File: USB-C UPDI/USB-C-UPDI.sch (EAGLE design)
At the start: 9 parts, among them IC1 FT232RL, J2 61300511121

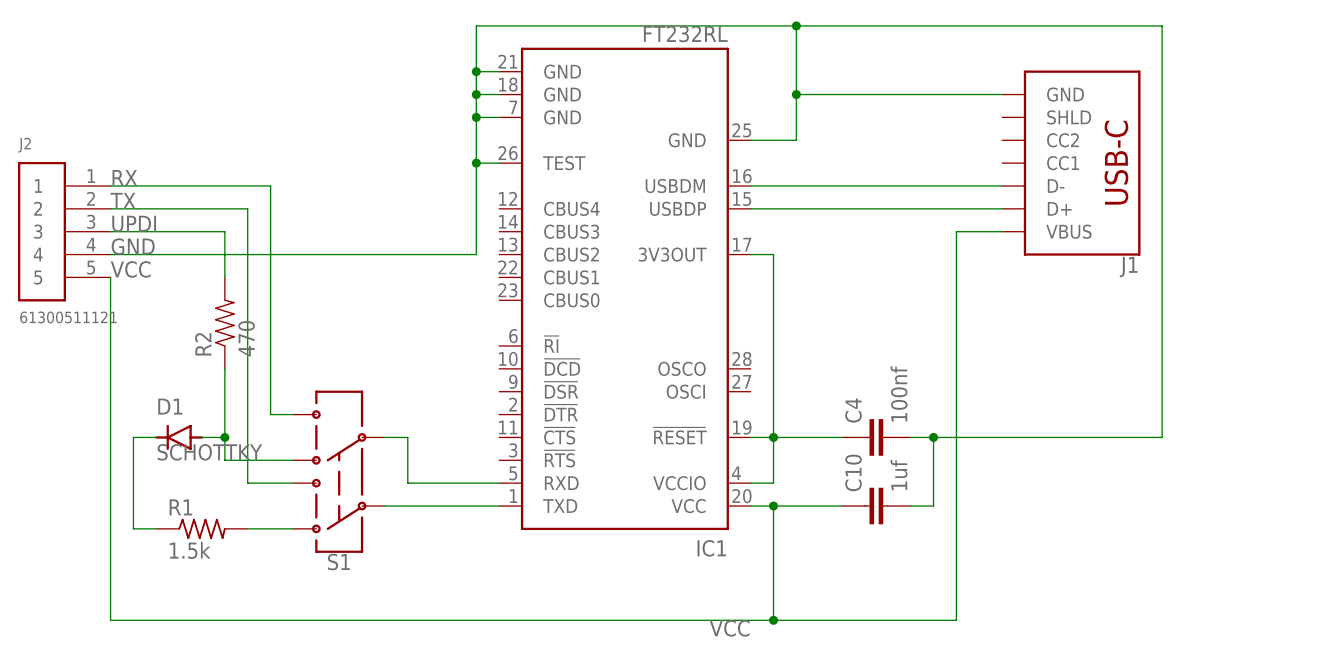
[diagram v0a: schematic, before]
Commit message: updates
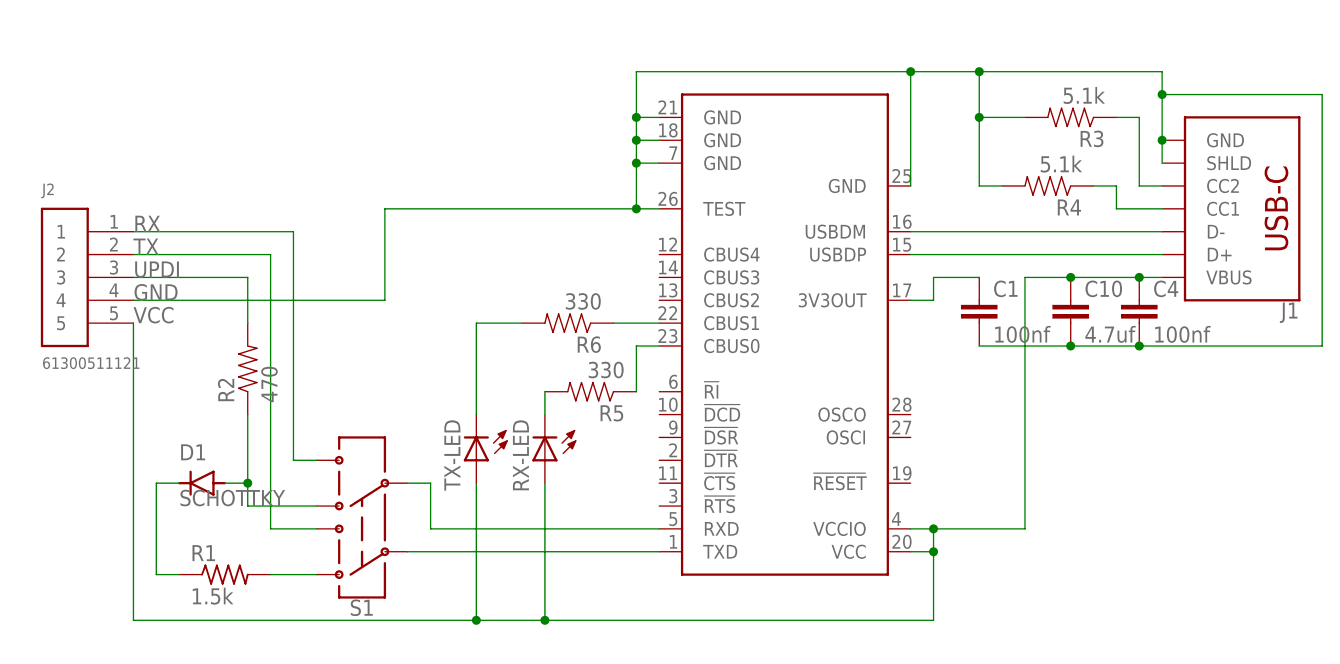
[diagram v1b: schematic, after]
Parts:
- added C1: 100nf, 01_SparkFun:CAP1206
- added R3, R4: 5.1k, 01_SparkFun:RESISTOR1206
- added R5, R6: 330, 01_SparkFun:RESISTOR1206
- added RX-LED, TX-LED: LED, eagle_fab:LED
- C10: value 1uf -> 4.7uf
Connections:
- new net N$1: C1.1, IC1.3V3OUT
- new net N$42: J1.CC2, R3.1
- new net N$43: IC1.CBUS1, R6.1
- new net N$44: IC1.CBUS0, R5.1
- new net N$45: R5.2, RX-LED.C
- new net N$46: R6.2, TX-LED.C
- net GND: now also C1.2, J1.SHLD, R3.2, R4.2
- net N$9: now also J1.CC1, R4.1; no longer C4.1, IC1.!RESET, IC1.3V3OUT, IC1.VCCIO
- net VCC: now also C4.1, IC1.VCCIO, RX-LED.A, TX-LED.A
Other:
- moved on the sheet: C10, C4, D1, J1, J2, R1, R2, S1
